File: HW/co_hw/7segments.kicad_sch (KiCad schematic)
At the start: 8 parts, among them U2 74HC595, U3 74HC595, U4 74HC595, U5 74HC595

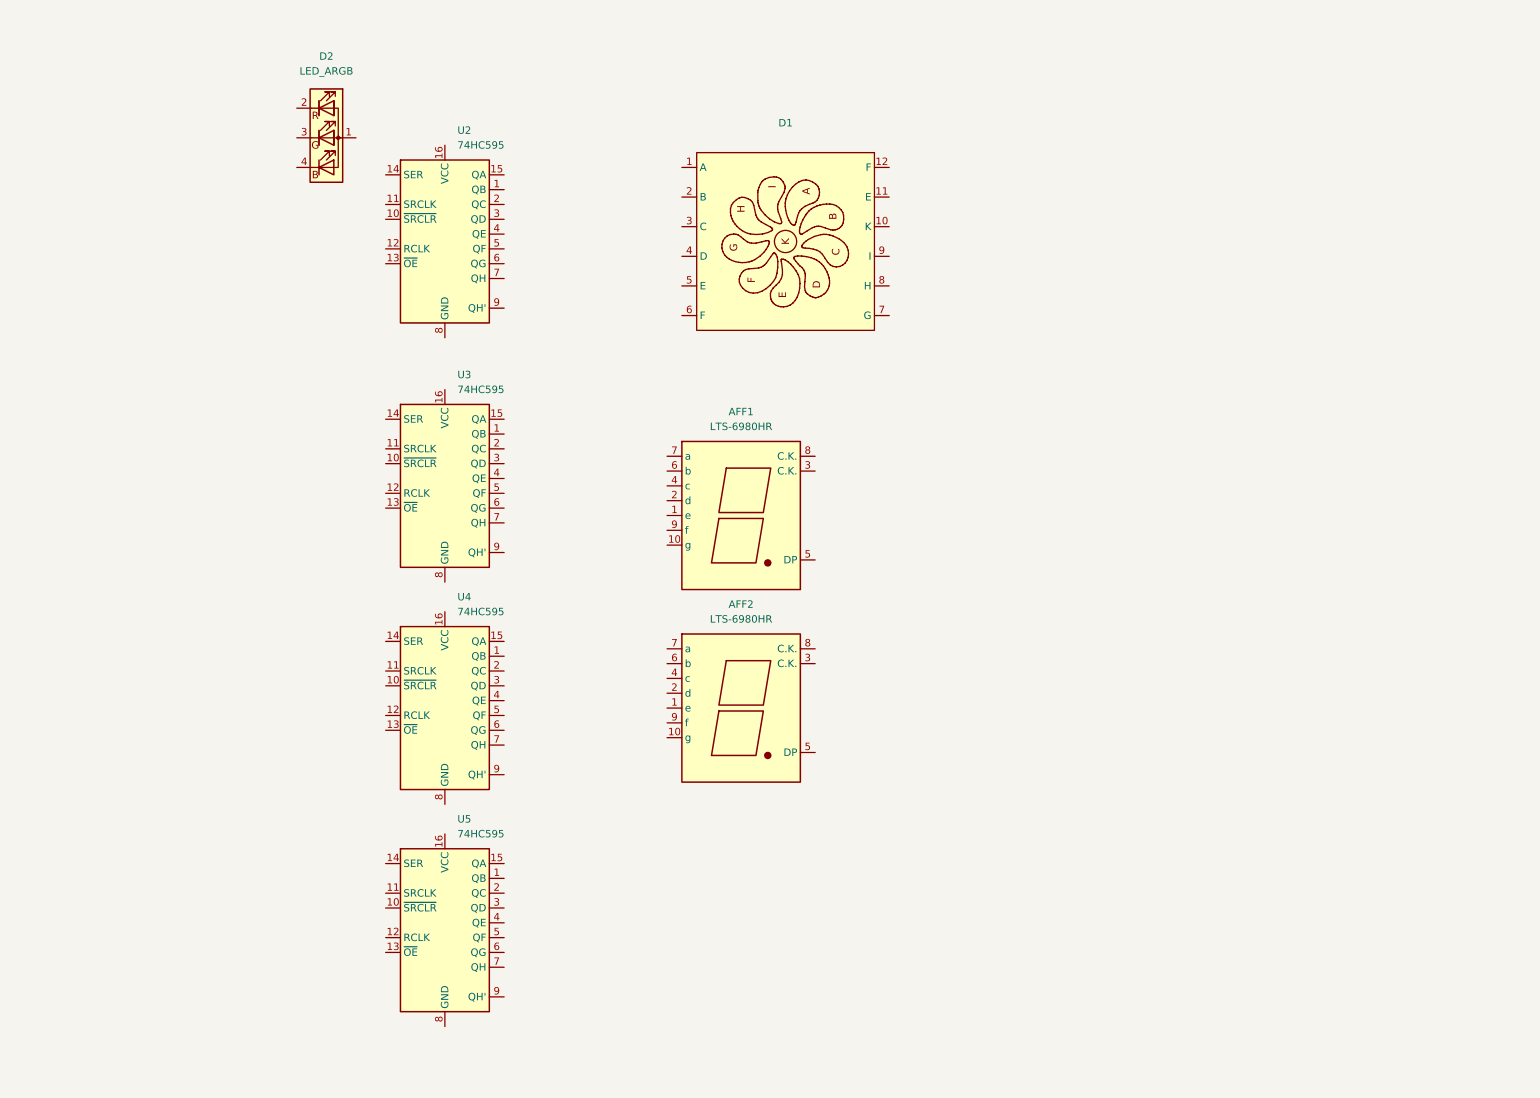
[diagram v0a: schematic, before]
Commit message: HW update.
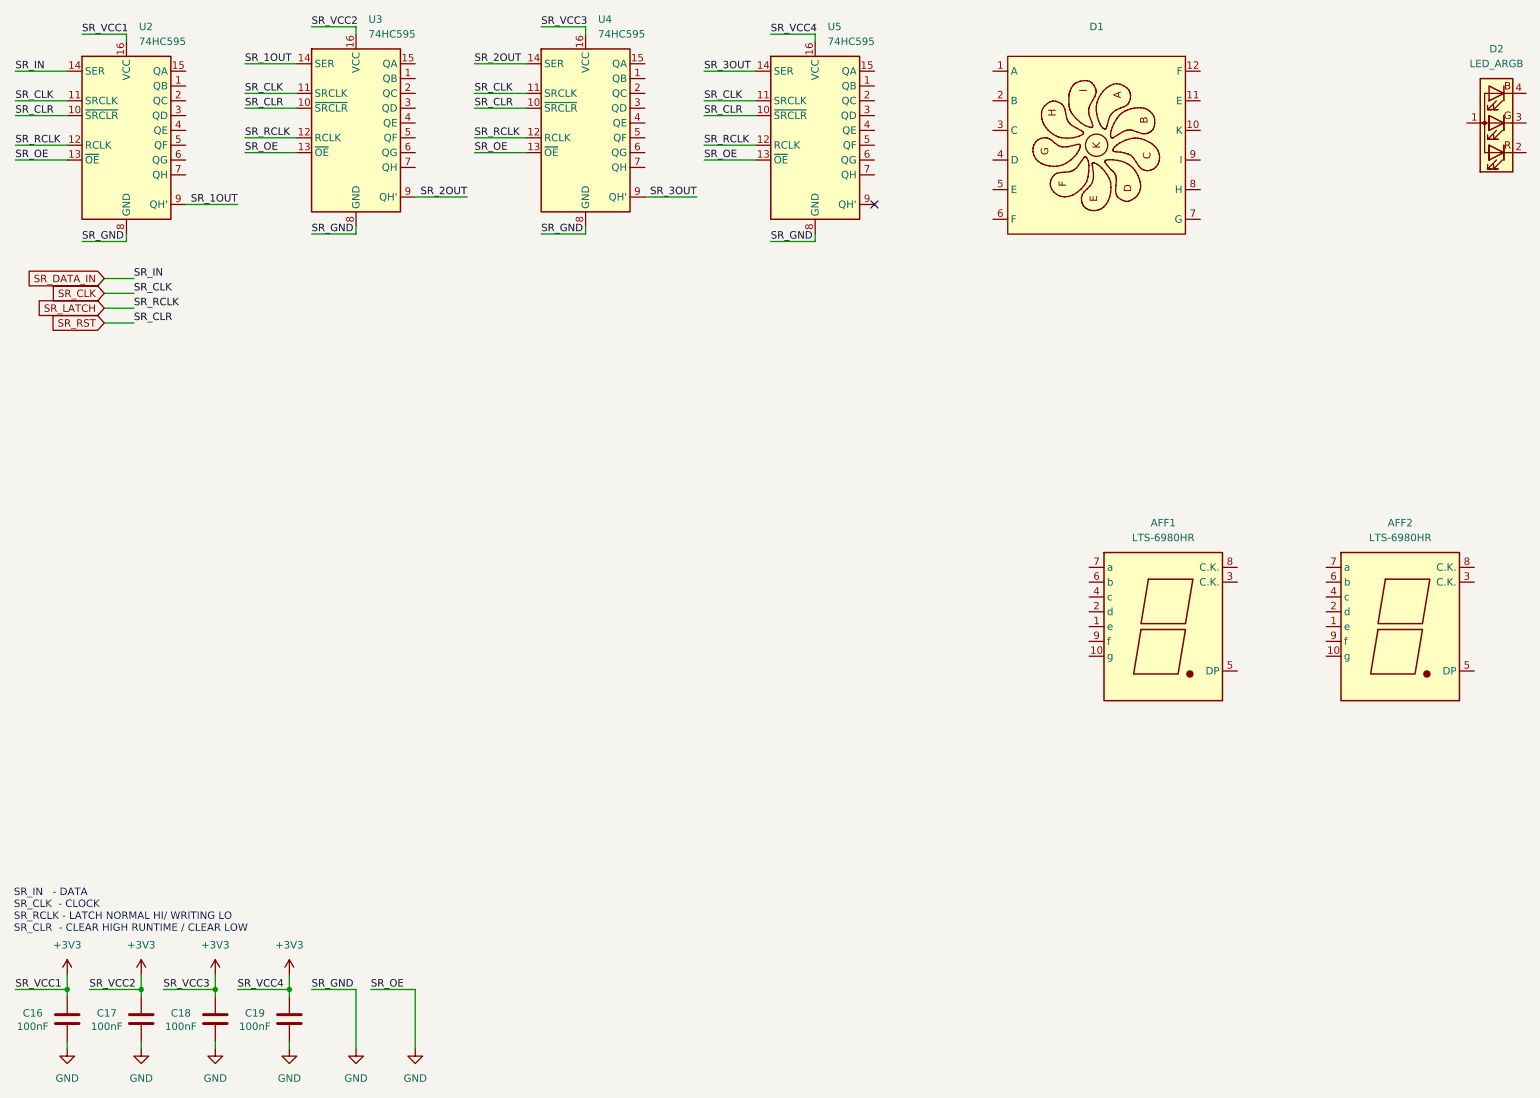
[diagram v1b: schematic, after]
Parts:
- added C16, C17, C18, C19: 100nF, symbol Device:C
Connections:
- net SR_RST: now reaches U4.10 (~{SRCLR})
- net SR_RST: now also U2.10 (~{SRCLR}), U3.10 (~{SRCLR}), U5.10 (~{SRCLR})
- net SR_CLK: now reaches U4.11 (SRCLK)
- net SR_CLK: now also U2.11 (SRCLK), U3.11 (SRCLK), U5.11 (SRCLK)
- net SR_LATCH: now reaches U4.12 (RCLK)
- net SR_LATCH: now also U2.12 (RCLK), U3.12 (RCLK), U5.12 (RCLK)
- net GND: now reaches U4.13 (~{OE})
- net GND: now also U2.13 (~{OE}), U2.8 (GND), U3.13 (~{OE}), U3.8 (GND), U4.8 (GND), U5.13 (~{OE}), U5.8 (GND), C16.2, C17.2, C18.2, C19.2
- net SR_2OUT: now reaches U4.14 (SER)
- net SR_2OUT: now also U3.9 (QH')
- net +3V3: now reaches U4.16 (VCC)
- net +3V3: now also U2.16 (VCC), U3.16 (VCC), U5.16 (VCC), C16.1, C17.1, C18.1, C19.1
- net SR_3OUT: now reaches U4.9 (QH')
- net SR_3OUT: now also U5.14 (SER)
- net SR_1OUT: now reaches U3.14 (SER)
- net SR_1OUT: now also U2.9 (QH')
- net SR_DATA_IN: now reaches U2.14 (SER)
- no-connect marks 0 -> 1
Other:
- note added: "SR_IN - DATA SR_CLK - CLOCK SR_RCLK - LATCH NORMAL HI/ WRITING LO SR_CLR - CLEAR HIGH RUNTIME / CLEAR LOW"
- moved on the sheet: AFF1, AFF2, D1, D2, U2, U3, U4, U5
